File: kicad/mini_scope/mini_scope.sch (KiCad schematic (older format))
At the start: 7 parts

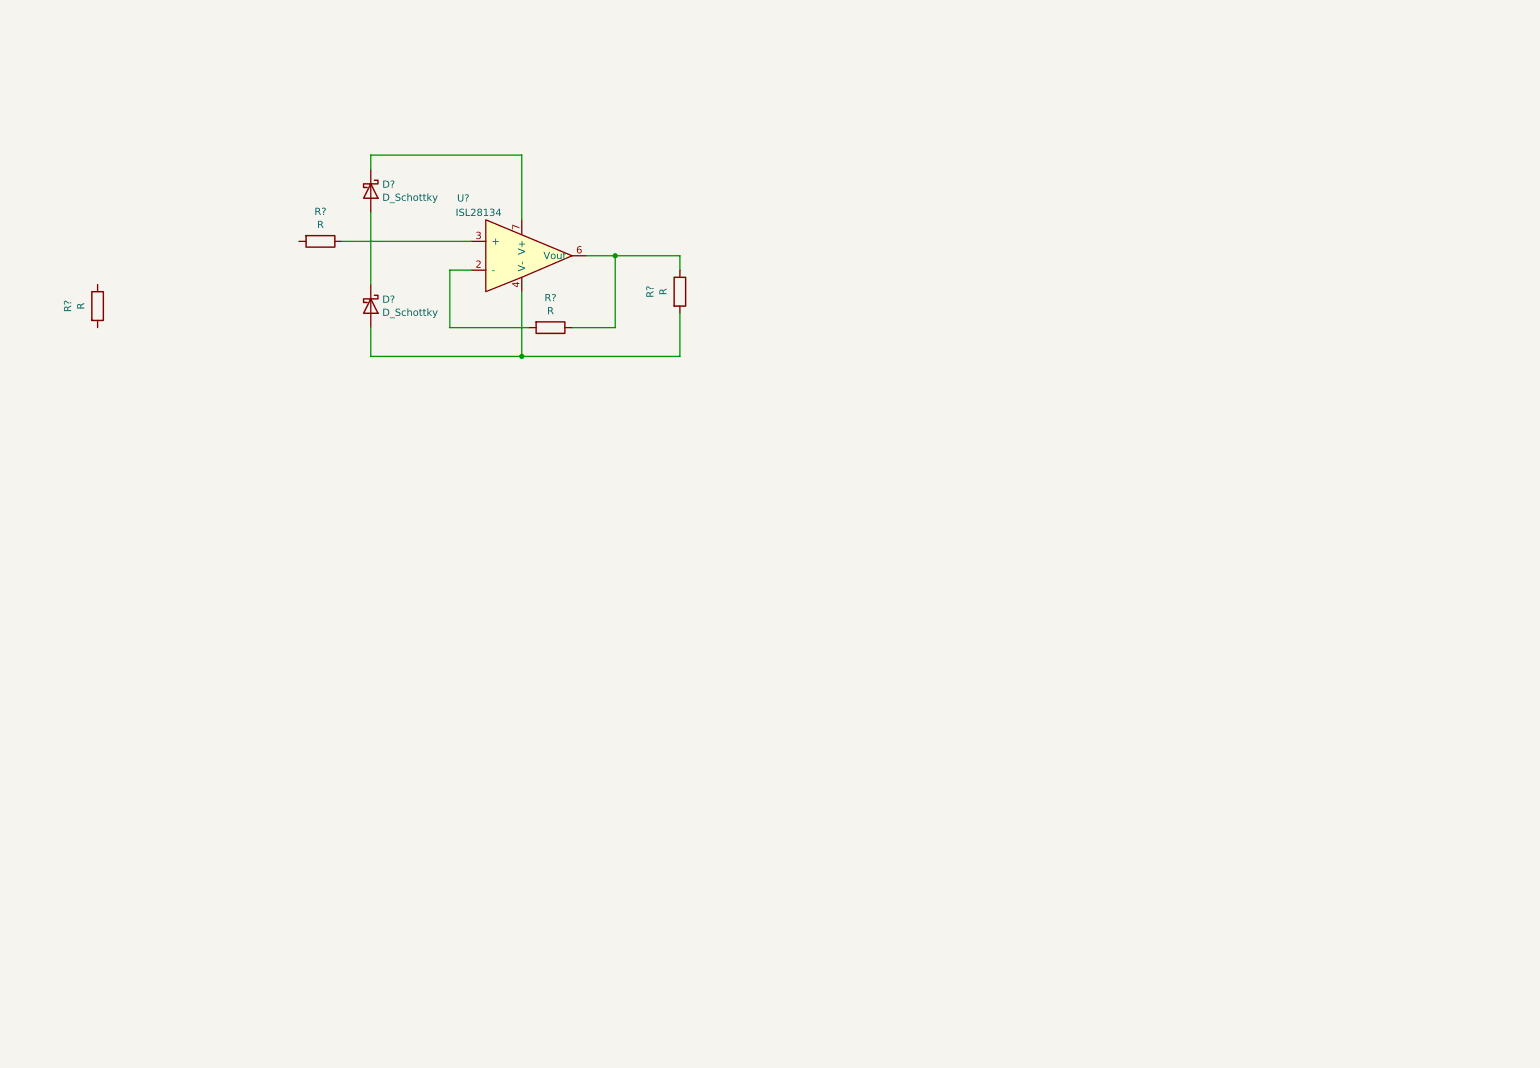
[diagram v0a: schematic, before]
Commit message: schematic complete
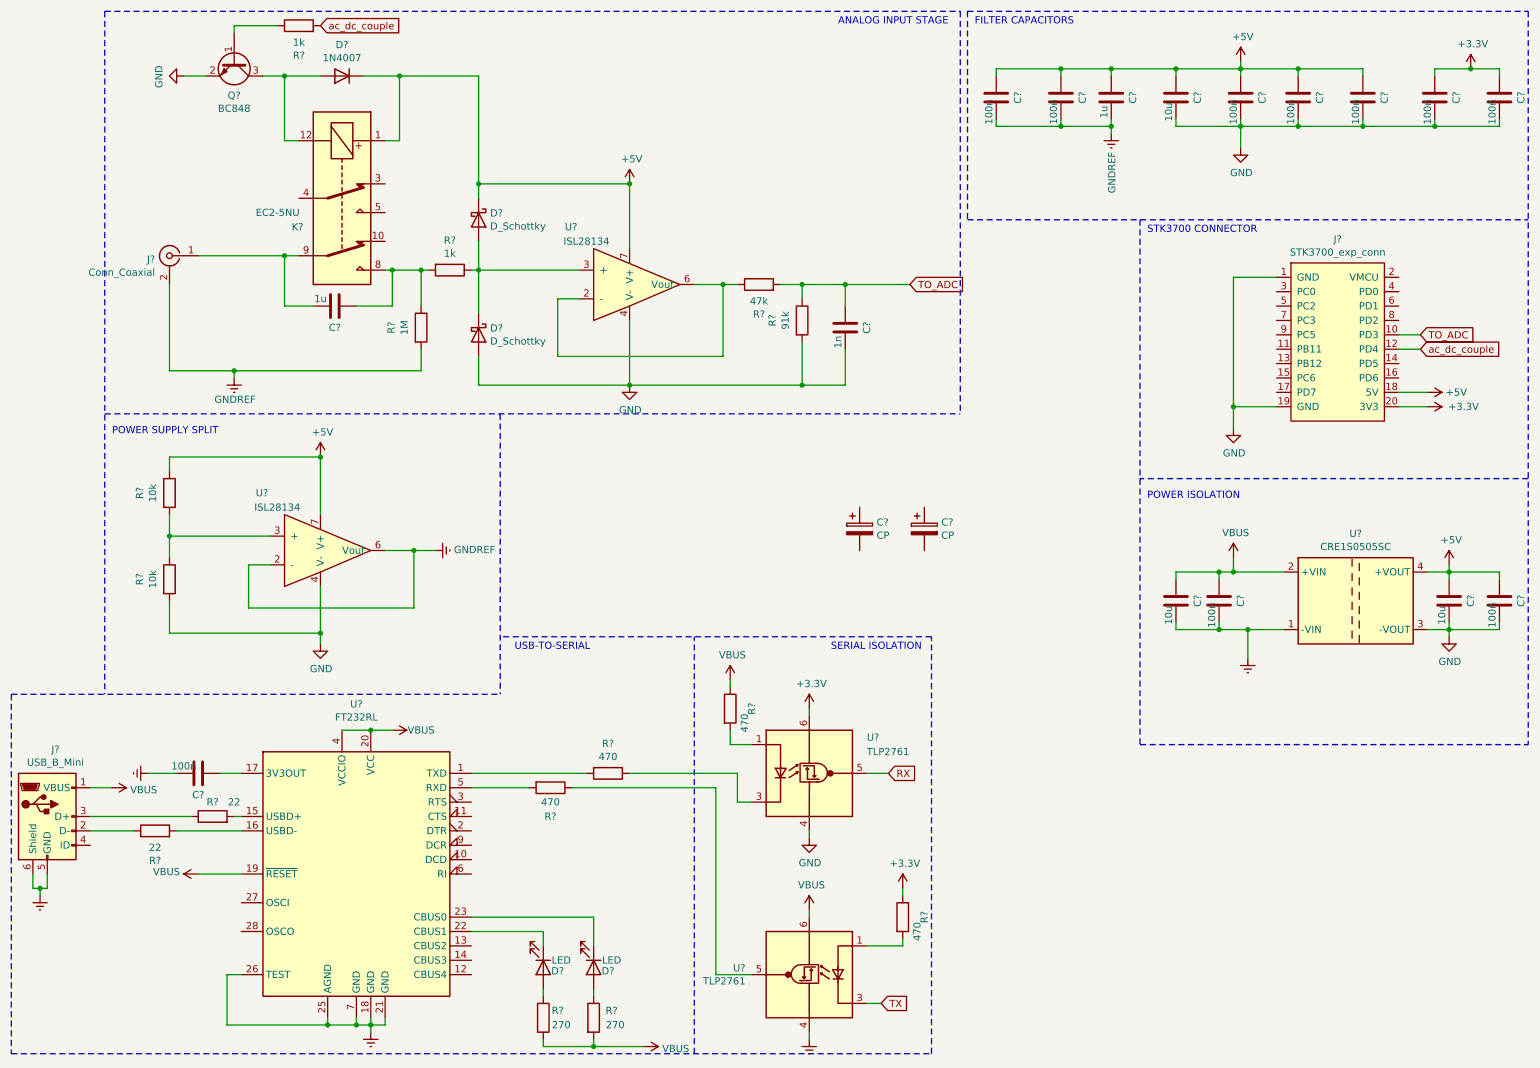
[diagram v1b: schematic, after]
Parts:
- removed R?: R, symbol Device:R
- added C? (x2): 1u, symbol Device:C
- added C?: 1n, symbol Device:C
- added C? (x3): 10u, symbol Device:C
- added C? (x10): 100n, symbol Device:C
- added C? (x2): CP, symbol Device:CP
- added D?: 1N4007, Diode_THT:D_DO-41_SOD81_P10.16mm_Horizontal, symbol Diode:1N4007
- added D? (x2): LED, symbol Device:LED
- added J?: Conn_Coaxial, symbol Connector:Conn_Coaxial
- added J?: STK3700_exp_conn, symbol conn:STK3700_exp_conn
- added J?: USB_B_Mini, symbol Connector:USB_B_Mini
- added K?: EC2-5NU, Relay_THT:Relay_DPDT_Kemet_EC2, symbol Relay:EC2-5NU
- added Q?: BC848, Package_TO_SOT_SMD:SOT-23, symbol Transistor_BJT:BC848
- added R? (x2): 10k, symbol Device:R
- added R?: 1k, symbol Device:R
- added R?: 91k, symbol Device:R
- added R? (x2): 22, symbol Device:R
- added R? (x4): 470, symbol Device:R
- added R? (x2): 270, symbol Device:R
- added U?: ISL28134, symbol lib1:ISL28134
- added U?: FT232RL, Package_SO:SSOP-28_5.3x10.2mm_P0.65mm, symbol Interface_USB:FT232RL
- added U?: CRE1S0505SC, Converter_DCDC:Converter_DCDC_muRata_CRE1xxxxxxSC_THT, symbol Regulator_Switching:CRE1S0505SC
- added U? (x2): TLP2761, Package_SO:SO-6L_10x3.84mm_P1.27mm, symbol Isolator:TLP2761
- R?: value R -> 1k
- R?: value R -> 47k
- R?: value R -> 1M
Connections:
- net at U?.2 (-): now also R?.1, U?.6 (Vout)
- net at R?.1, U?.3 (+): now also D?.1 (K), D?.2 (A)
- net GND: now reaches D?.2 (A), U?.4 (V-)
- net GND: now also C?.2, C?.2, C?.2, C?.2, C?.2, C?.2, C?.2, C?.2, C?.2, J?.1 (GND), J?.19 (GND), Q?.2 (E), R?.2, R?.2, U?.3 (-VOUT), U?.4 (GND), U?.4 (V-); no longer R?.2
- net +5V: now reaches D?.1 (K), U?.7 (V+)
- net +5V: now also C?.1, C?.1, C?.1, C?.1, C?.1, C?.1, C?.1, C?.1, C?.1, D?.1 (K), J?.18 (5V), K?.1, R?.1, U?.4 (+VOUT), U?.7 (V+)
- net at R?.2: now also R?.1, C?.1, K?.8
- net GNDREF: now reaches R?.2
- net GNDREF: now also C?.2, C?.2, C?.2, J?.2 (Ext), U?.2 (-), U?.6 (Vout)
- new net: R?.1, R?.2, U?.3 (+)
- new net: C?.2, J?.1 (In), K?.9
- new net: Q?.1 (B), R?.1
- new net: D?.2 (A), K?.12, Q?.3 (C)
- new net: R?.2, U?.1 (TXD)
- new net: R?.2, U?.15 (USBD+)
- new net: R?.2, U?.16 (USBD-)
- new net: C?.1, U?.17 (3V3OUT)
- new net: D?.1 (K), U?.22 (CBUS1)
- new net: D?.1 (K), U?.23 (CBUS0)
- new net: R?.2, U?.5 (RXD)
- new net: J?.3 (D+), R?.1
- new net: J?.2 (D-), R?.1
- new net: R?.1, U?.5 (VO)
- new net: R?.1, U?.3 (K)
- new net: R?.2, U?.1 (A) (x2)
- new net: D?.2 (A), R?.1 (x2)
- new net +3V3: C?.1, C?.1, J?.20 (3V3), R?.1, U?.6 (VDD)
- new net Earth: C?.2, C?.2, C?.2, J?.5 (GND), J?.6 (Shield), U?.1 (-VIN), U?.18 (GND), U?.21 (GND), U?.25 (AGND), U?.26 (TEST), U?.4 (GND), U?.7 (GND)
- new net RX: U?.5 (VO)
- new net TO_ADC: C?.1, J?.10 (PD3), R?.1, R?.2
- new net TX: U?.3 (K)
- new net VBUS: C?.1, C?.1, J?.1 (VBUS), R?.1, R?.2, R?.2, U?.19 (~RESET~), U?.2 (+VIN), U?.20 (VCC), U?.4 (VCCIO), U?.6 (VDD)
- new net ac_dc_couple: J?.12 (PD4), R?.2
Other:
- note added: "ANALOG INPUT STAGE\n"
- note added: "FILTER CAPACITORS\n"
- note added: "POWER ISOLATION\n"
- note added: "POWER SUPPLY SPLIT\n"
- note added: "SERIAL ISOLATION"
- note added: "STK3700 CONNECTOR\n"
- note added: "USB-TO-SERIAL"
- moved on the sheet: D?, R?, U?
